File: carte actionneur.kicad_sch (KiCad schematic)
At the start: 47 parts, among them J1 Conn_01x03_Pin, J10 Conn_01x03_Pin, J11 Conn_01x02, J12 Screw_Terminal_01x02, J13 Screw_Terminal_01x02, J14 Screw_Terminal_01x02, J15 Conn_01x02, J2 Conn_01x02, J3 Conn_01x03_Pin, J4 Conn_01x03_Pin, J4 Connecteur Programmation, J6 Conn_01x03_Pin, J7 Conn_01x03_Pin, J8 Conn_01x03_Pin, J9 Conn_01x03_Pin, Q1 BSS83P, Q2 2N7000, U1 MEGA_PRO_EMBED_CH340G___ATMEG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, U2 LM317_TO-252, U3 ZXBM5210-SP, U4 YAAJ_DCDC_StepDown_LM2596, U5 YAAJ_DCDC_StepDown_LM2596, U6 YAAJ_DCDC_StepDown_LM2596, U7 ZXBM5210-SP

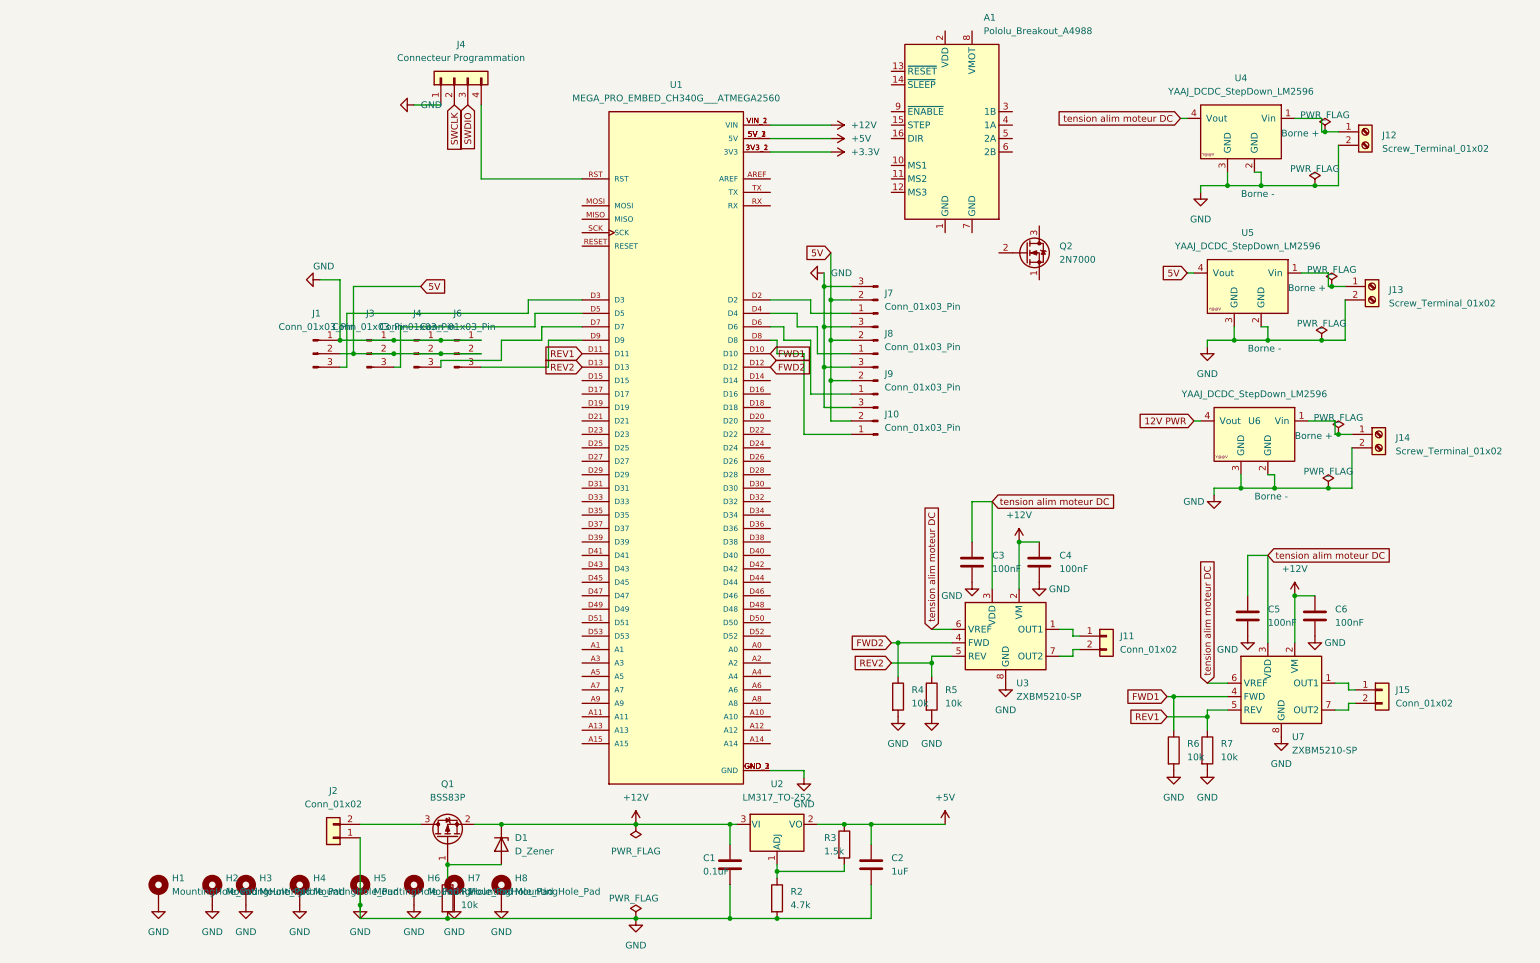
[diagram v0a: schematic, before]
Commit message: test git
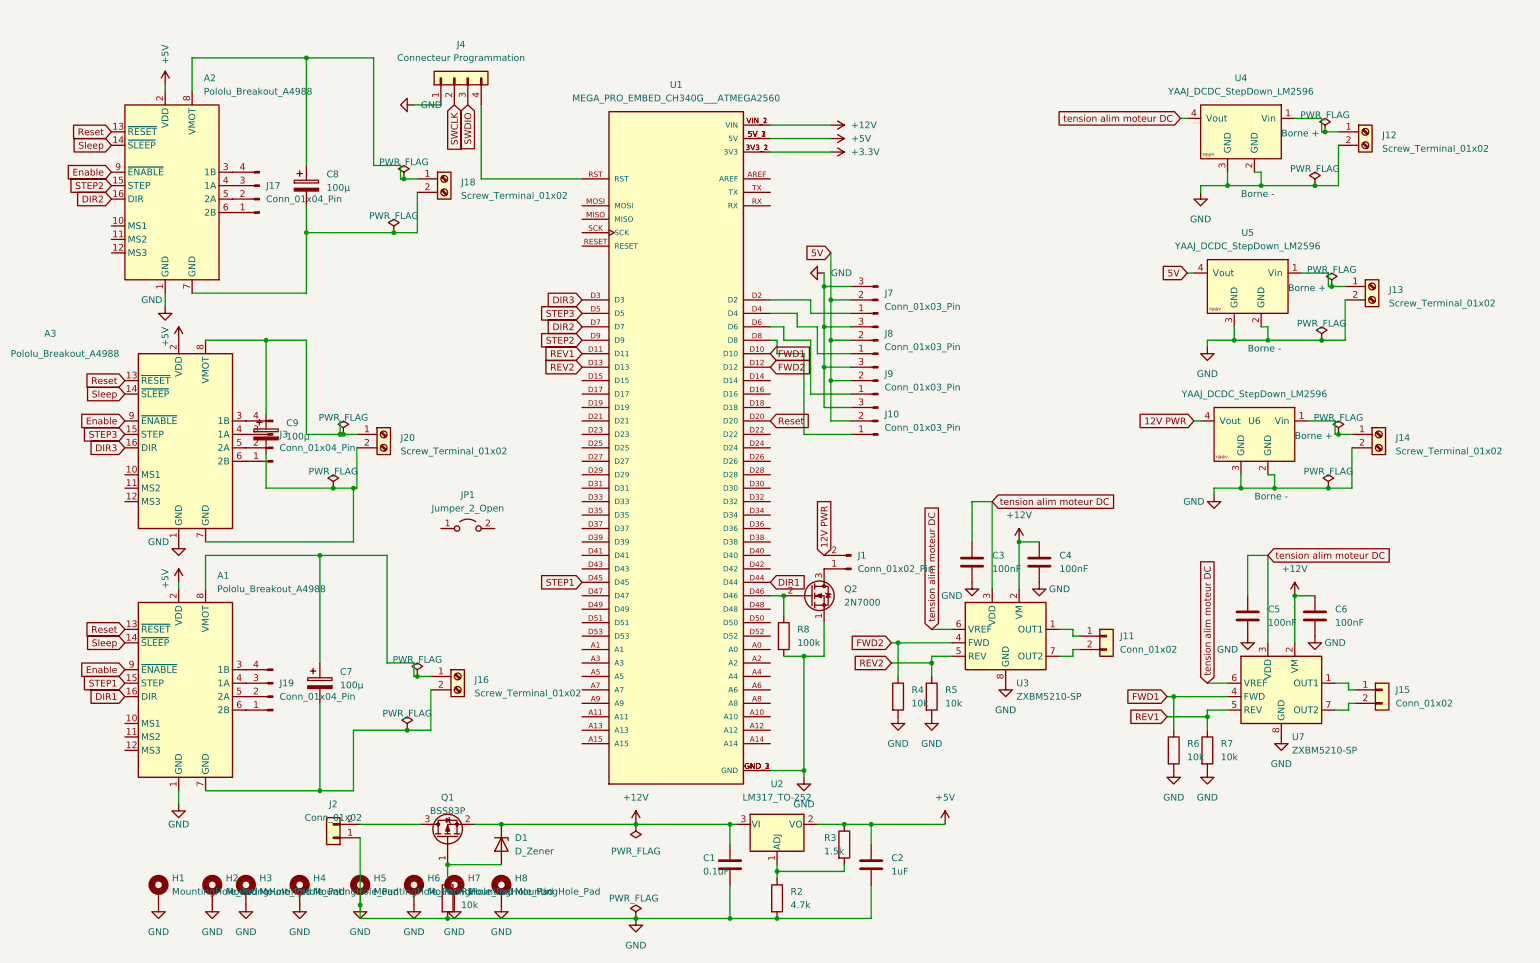
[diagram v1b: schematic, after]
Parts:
- removed J1, J3, J4, J6: Conn_01x03_Pin, Connector_PinHeader_2.54mm:PinHeader_1x03_P2.54mm_Vertical, symbol Connector:Conn_01x03_Pin
- added A2, A3: Pololu_Breakout_A4988, Module:Pololu_Breakout-16_15.2x20.3mm, symbol Driver_Motor:Pololu_Breakout_A4988
- added C7, C8, C9: 100µ, symbol Device:C_Polarized
- added J1: Conn_01x02_Pin, Connector_PinHeader_2.54mm:PinHeader_1x03_P2.54mm_Vertical, symbol Connector:Conn_01x02_Pin
- added J16, J18, J20: Screw_Terminal_01x02, TerminalBlockBend:CUI_TBP01R1-508-02BE, symbol Connector:Screw_Terminal_01x02
- added J17, J19, J3: Conn_01x04_Pin, Connector_JST:JST_XH_B4B-XH-A_1x04_P2.50mm_Vertical, symbol Connector:Conn_01x04_Pin
- added JP1: Jumper_2_Open, Jumper:SolderJumper-2_P1.3mm_Open_TrianglePad1.0x1.5mm, symbol Jumper:Jumper_2_Open
- added R8: 100k, Resistor_SMD:R_0805_2012Metric, symbol Device:R
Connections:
- net +5V: now also A1.2 (VDD), A2.2 (VDD), A3.2 (VDD)
- net 12V PWR: now also J1.2 (Pin_2)
- net GND: now also A1.1 (GND), Q2.1 (S), A2.1 (GND), A3.1 (GND), R8.2
- net Reset: now reaches A1.13 (~{RESET})
- net Reset: now also U1.D20, A2.13 (~{RESET}), A3.13 (~{RESET})
- net Sleep: now reaches A1.14 (~{SLEEP})
- net Sleep: now also A2.14 (~{SLEEP}), A3.14 (~{SLEEP})
- net STEP1: now reaches A1.15 (STEP)
- net STEP1: now also U1.D45
- net DIR1: now reaches A1.16 (DIR)
- net DIR1: now also U1.D44
- net at A1.3 (1B): now also J19.4 (Pin_4)
- net at A1.4 (1A): now also J19.3 (Pin_3)
- net at A1.5 (2A): now also J19.2 (Pin_2)
- net at A1.6 (2B): now also J19.1 (Pin_1)
- net at A1.7 (GND): now also C7.2, J16.2 (Pin_2)
- net at A1.8 (VMOT): now also C7.1, J16.1 (Pin_1)
- net Enable: now reaches A1.9 (~{ENABLE})
- net Enable: now also A2.9 (~{ENABLE}), A3.9 (~{ENABLE})
- net DIR3: now reaches U1.D3
- net DIR3: now also A3.16 (DIR)
- net at U1.D46: now also Q2.2 (G), R8.1
- net STEP3: now reaches U1.D5
- net STEP3: now also A3.15 (STEP)
- net DIR2: now reaches U1.D7
- net DIR2: now also A2.16 (DIR)
- net STEP2: now reaches U1.D9
- net STEP2: now also A2.15 (STEP)
- net at Q2.3 (D): now also J1.1 (Pin_1)
- new net: A2.6 (2B), J17.1 (Pin_1)
- new net: A2.5 (2A), J17.2 (Pin_2)
- new net: A2.4 (1A), J17.3 (Pin_3)
- new net: A2.3 (1B), J17.4 (Pin_4)
- new net: A2.8 (VMOT), C8.1, J18.1 (Pin_1)
- new net: A2.7 (GND), C8.2, J18.2 (Pin_2)
- new net: A3.8 (VMOT), C9.1, J20.1 (Pin_1)
- new net: A3.7 (GND), C9.2, J20.2 (Pin_2)
- new net: A3.3 (1B), J3.4 (Pin_4)
- new net: A3.4 (1A), J3.3 (Pin_3)
- new net: A3.5 (2A), J3.2 (Pin_2)
- new net: A3.6 (2B), J3.1 (Pin_1)
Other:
- moved on the sheet: A1, Q2
